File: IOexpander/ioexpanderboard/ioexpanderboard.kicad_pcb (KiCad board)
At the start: 2 copper layers, 33 x 63.5 mm, 12 parts, among them U1 ATtiny44-20PU, U2 74LVC245, U3 LD1117S33TR_SOT223

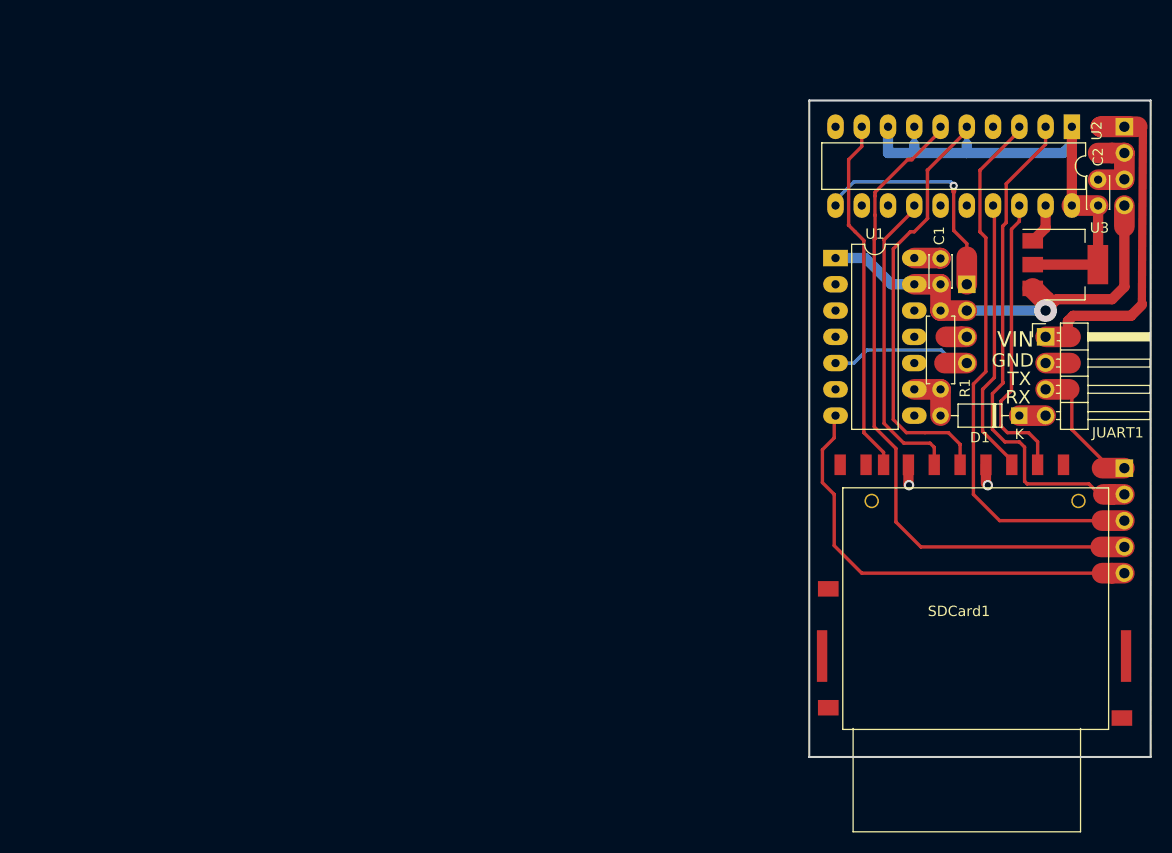
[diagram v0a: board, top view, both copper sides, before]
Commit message: Production files for cpu board. More work on IO expander board
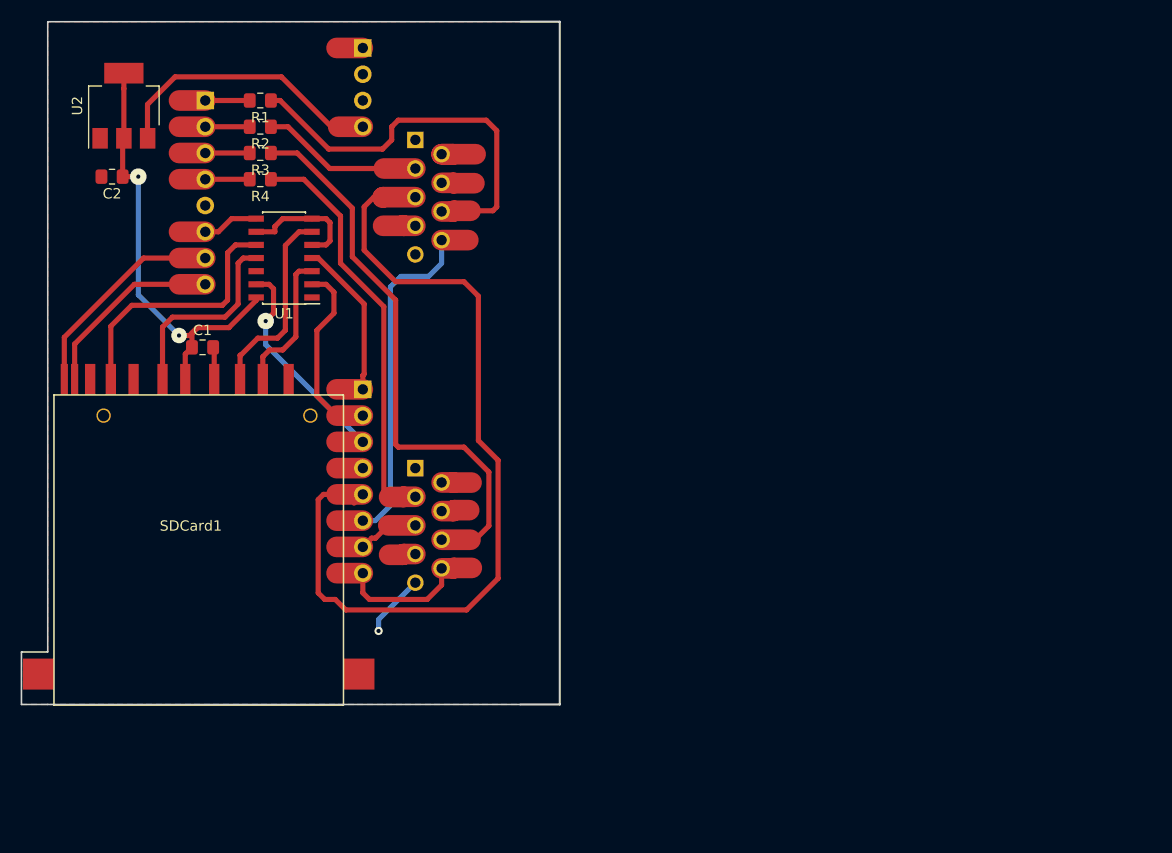
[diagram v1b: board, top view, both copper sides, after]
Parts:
- removed D1: 1N4148, Diode_THT:D_DO-35_SOD27_P7.62mm_Horizontal
- removed JIN1, JPOWER2: Conn_01x04_Male, Connector_PinHeader_2.54mm:PinHeader_1x04_P2.54mm_Vertical
- removed JOUT1: Conn_01x05_Male, Connector_PinHeader_2.54mm:PinHeader_1x05_P2.54mm_Vertical
- removed JUART1: Conn_01x04_Male, Connector_PinHeader_2.54mm:PinHeader_1x04_P2.54mm_Horizontal
- removed U3: LD1117S33TR_SOT223, Package_TO_SOT_SMD:SOT-223-3_TabPin2
- added JINPUT1: Conn_01x08_Male, Connector_PinHeader_2.54mm:PinHeader_1x08_P2.54mm_Vertical, B.Cu at (111.8, 63.5)
- added JOUTPUT1: Conn_01x08_Male, Connector_PinHeader_2.54mm:PinHeader_1x08_P2.54mm_Vertical, B.Cu at (127.0, 91.4)
- added JPOWER1: Conn_01x04_Male, Connector_PinHeader_2.54mm:PinHeader_1x04_P2.54mm_Vertical, B.Cu at (127.0, 58.4)
- added JSERIAL1: DB9_Male, Connector_Dsub:DSUB-9_Male_Horizontal_P2.77x2.54mm_EdgePinOffset9.40mm, B.Cu at (132.1, 67.3)
- added JSERIAL2: DB9_Male, Connector_Dsub:DSUB-9_Male_Horizontal_P2.77x2.54mm_EdgePinOffset9.40mm, B.Cu at (132.1, 99.1)
- added R2: 330, Resistor_SMD:R_0805_2012Metric_Pad1.15x1.40mm_HandSolder, F.Cu at (117.1, 66.0)
- added R3: 330, Resistor_SMD:R_0805_2012Metric_Pad1.15x1.40mm_HandSolder, F.Cu at (117.1, 68.6)
- added R4: 330, Resistor_SMD:R_0805_2012Metric_Pad1.15x1.40mm_HandSolder, F.Cu at (117.1, 71.1)
- C1: footprint Capacitor_THT:C_Disc_D3.0mm_W2.0mm_P2.50mm -> Capacitor_SMD:C_0805_2012Metric_Pad1.15x1.40mm_HandSolder
- C2: value 100nF -> 10uF; footprint Capacitor_THT:C_Disc_D3.0mm_W2.0mm_P2.50mm -> Capacitor_SMD:C_0805_2012Metric_Pad1.15x1.40mm_HandSolder
- R1: value 10k -> 330; footprint Resistor_THT:R_Axial_DIN0207_L6.3mm_D2.5mm_P7.62mm_Horizontal -> Resistor_SMD:R_0805_2012Metric_Pad1.15x1.40mm_HandSolder
- U1: value ATtiny44-20PU -> 74LVC86; footprint Package_DIP:DIP-14_W7.62mm_LongPads -> Package_SO:SOIC-14_3.9x8.7mm_P1.27mm
- U2: value 74LVC245 -> LD1117S33TR_SOT223; footprint Package_DIP:DIP-20_W7.62mm_LongPads -> Package_TO_SOT_SMD:SOT-223-3_TabPin2
- moved C2 95.4 mm to (102.7, 70.9), turned to 180 degrees
- moved U2 91.7 mm to (103.9, 64.0), turned to 90 degrees
- moved SDCard1 74.8 mm to (111.1, 94.0)
- moved C1 71.6 mm to (111.5, 87.4), turned to 0 degrees
- moved R1 68.9 mm to (117.1, 63.5), turned to 180 degrees
- moved U1 53.3 mm to (119.4, 78.7), turned to 180 degrees
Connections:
- C1 pad 1: +5V -> +3V3
- R1 pad 1: +5V -> Net-(JSERIAL1-Pad8)
- R1 pad 2: Net-(D1-Pad2) -> /RXD1
- SDCard1 pad 10: Net-(SDCard1-Pad10) -> /CARD_DETECT
- SDCard1 pad 11: Net-(SDCard1-Pad11) -> /WRITE_PROTECT
- SDCard1 pad 12: Net-(SDCard1-Pad12) -> GND
- SDCard1 pad 13: Net-(SDCard1-Pad13) -> GND
- U1 pad 1: +5V -> GND
- U1 pad 10: Net-(U1-Pad10) -> Net-(SDCard1-Pad7)
- U1 pad 11: Net-(U1-Pad11) -> Net-(SDCard1-Pad5)
- U1 pad 12: Net-(U1-Pad12) -> GND
- U1 pad 13: +5V -> /SCK
- U1 pad 14: GND -> +3V3
- U1 pad 2: Net-(U1-Pad2) -> /CS
- U1 pad 3: Net-(U1-Pad3) -> Net-(SDCard1-Pad1)
- U1 pad 4: Net-(U1-Pad4) -> /MOSI
- U1 pad 5: /RX2 -> GND
- U1 pad 6: Net-(U1-Pad6) -> Net-(SDCard1-Pad2)
- U1 pad 7: /RTS -> GND
- U1 pad 8: Net-(U1-Pad8) -> /MISO
- U1 pad 9: Net-(D1-Pad2) -> GND
- U2 pad 1: +3V3 -> GND
- U2 pad 2: /SS -> +3V3
- U2 pad 3: /MOSI -> +5V
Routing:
- net /TXD1: track 0.00 -> 86.3 mm
- net Net-(JSERIAL2-Pad8): track 0.00 -> 55.1 mm
- net /SS: track 48.7 -> 0.00 mm
- net +3V3: track 89.3 -> 43.2 mm, vias 0 -> 2
- net /RTS: track 42.7 -> 0.00 mm
- net /SCK: track 65.1 -> 23.4 mm, vias 0 -> 1
- net Net-(JSERIAL2-Pad2): track 0.00 -> 39.9 mm
- net Net-(JSERIAL1-Pad8): track 0.00 -> 39.0 mm
- net /RTS1: track 0.00 -> 37.7 mm
- net /MOSI: track 53.5 -> 17.7 mm
- net /VIN: track 35.8 -> 0.00 mm
- net +5V: track 48.2 -> 27.2 mm, vias 1 -> 0
- net /WRITE_PROTECT: track 0.00 -> 20.9 mm
- net /CARD_DETECT: track 0.00 -> 18.5 mm
- net /CS: track 0.00 -> 18.4 mm
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- added copper zone on F.Cu, net GND
- removed copper zone on F.Cu, net (none)
- removed copper zone on B.Cu, net GND
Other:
- board size 33 x 63.5 mm -> 52.1 x 66 mm
- board text removed: "GND"
- board text removed: "IO expander board for ByteMachine github.com /c0pperdragon /ByteMachine"
- board text removed: "RX"
- board text removed: "TX"
- board text removed: "VIN"
